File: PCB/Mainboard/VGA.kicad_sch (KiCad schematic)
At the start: 98 parts, among them J2 LCD_Connector, Q1 2SA1881-6, Q2 8C, U51 CHIPS65535

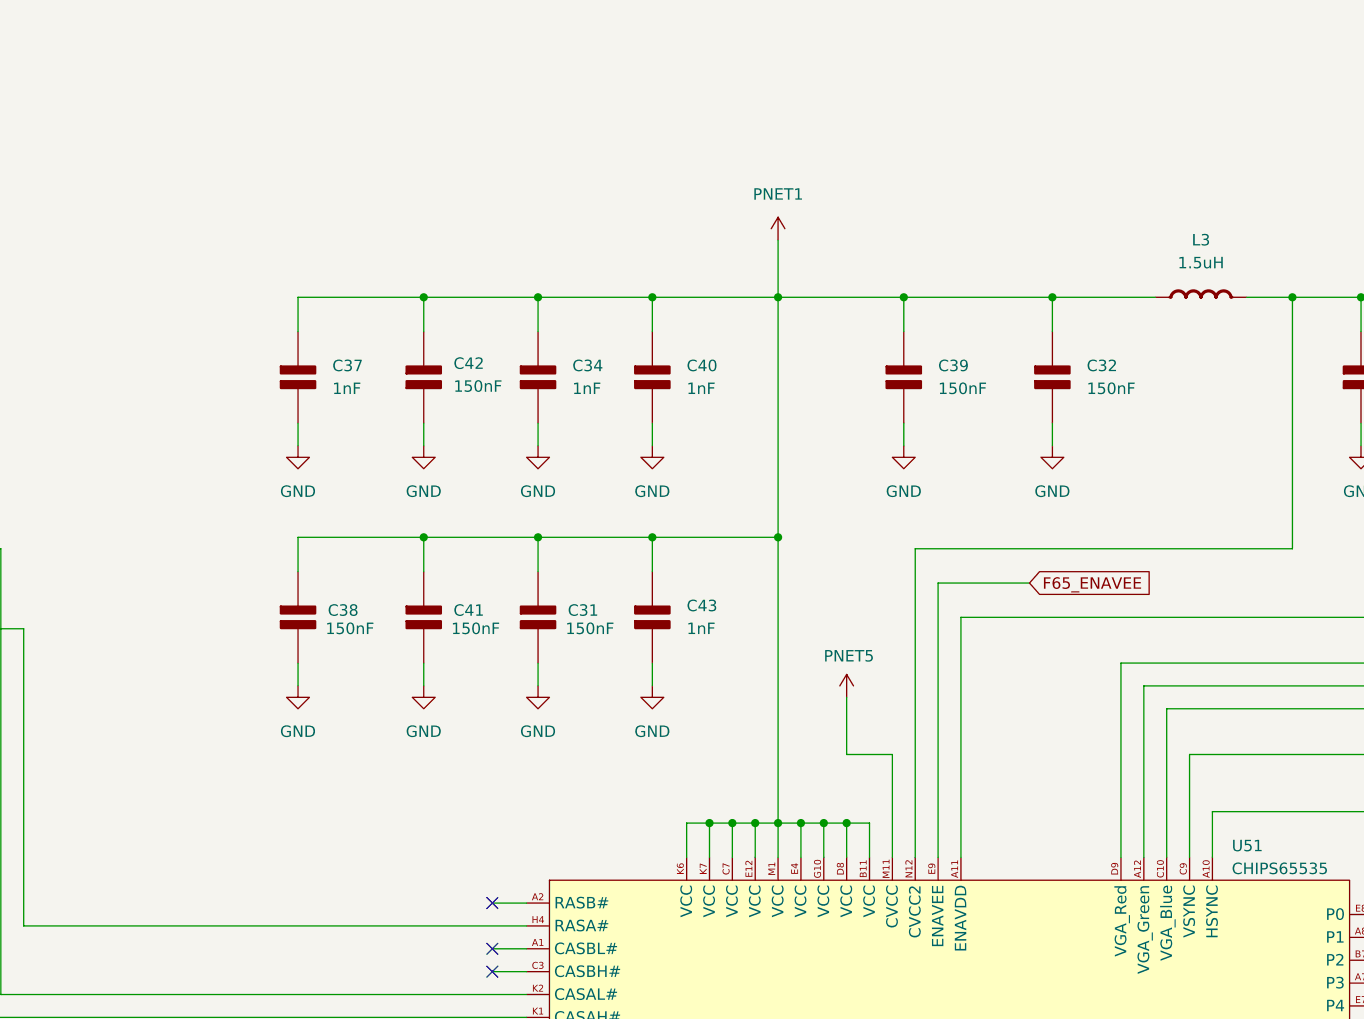
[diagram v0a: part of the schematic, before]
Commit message: Add files via upload
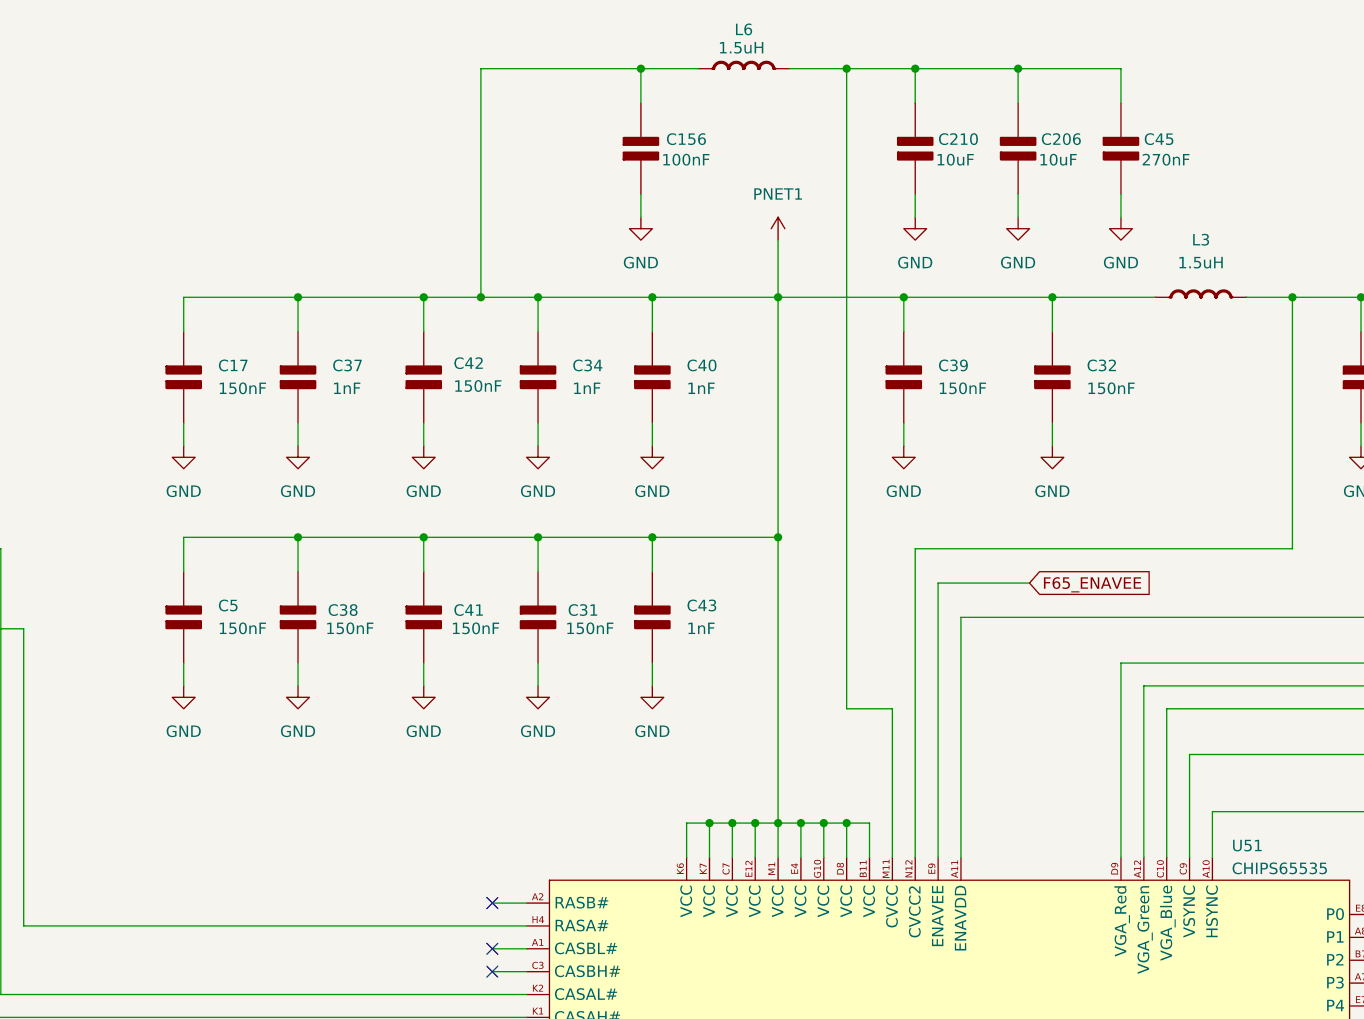
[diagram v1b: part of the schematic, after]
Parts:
- added C156: 100nF, symbol PCM_Elektuur:C
- added C17, C5: 150nF, symbol PCM_Elektuur:C
- added C206, C210: 10uF, symbol PCM_Elektuur:C
- added C45: 270nF, symbol PCM_Elektuur:C
- added L6: 1.5uH, symbol PCM_Elektuur:L
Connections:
- net GND: now also C156.1 (+), C17.2 (-), C206.2 (-), C210.2 (-), C45.2 (-), C5.2 (-)
- net PNET1: now also C156.2 (-), C17.1 (+), C5.1 (+), L6.2 (-)
- net PNET5: no longer U51.M11 (CVCC)
- new net: C206.1 (+), C210.1 (+), C45.1 (+), L6.1 (+), U51.M11 (CVCC)

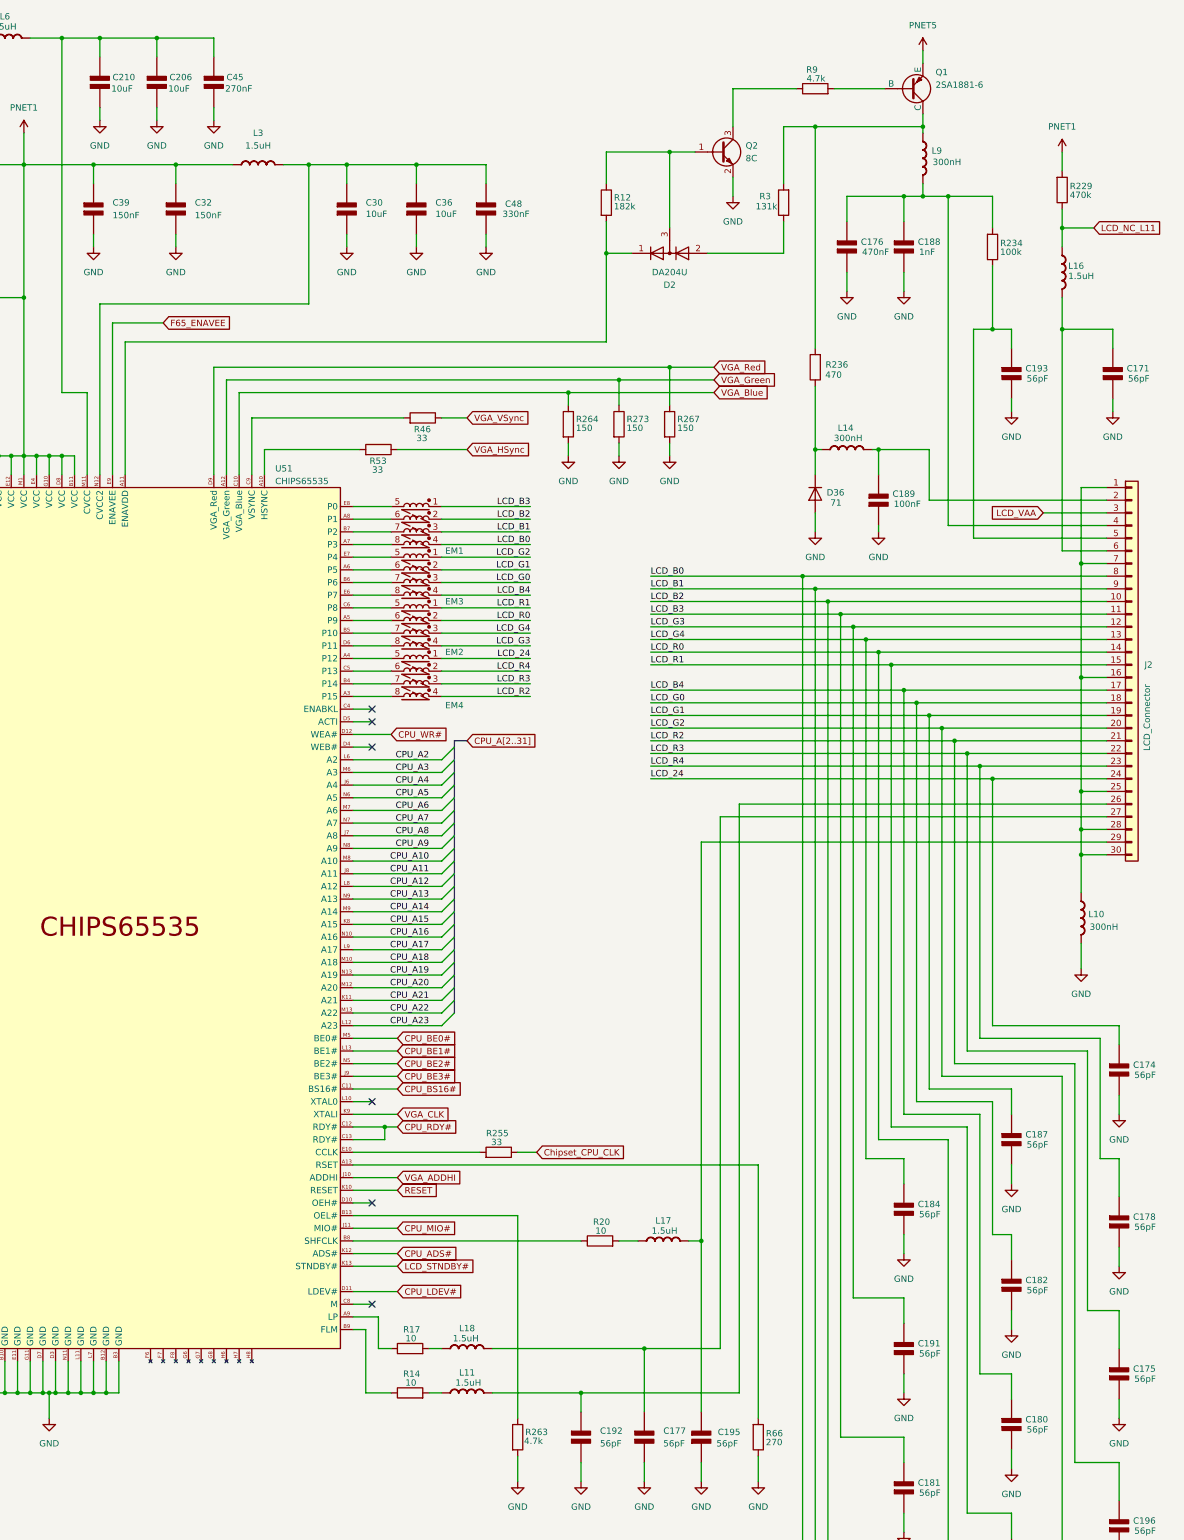
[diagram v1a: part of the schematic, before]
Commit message: Add files via upload
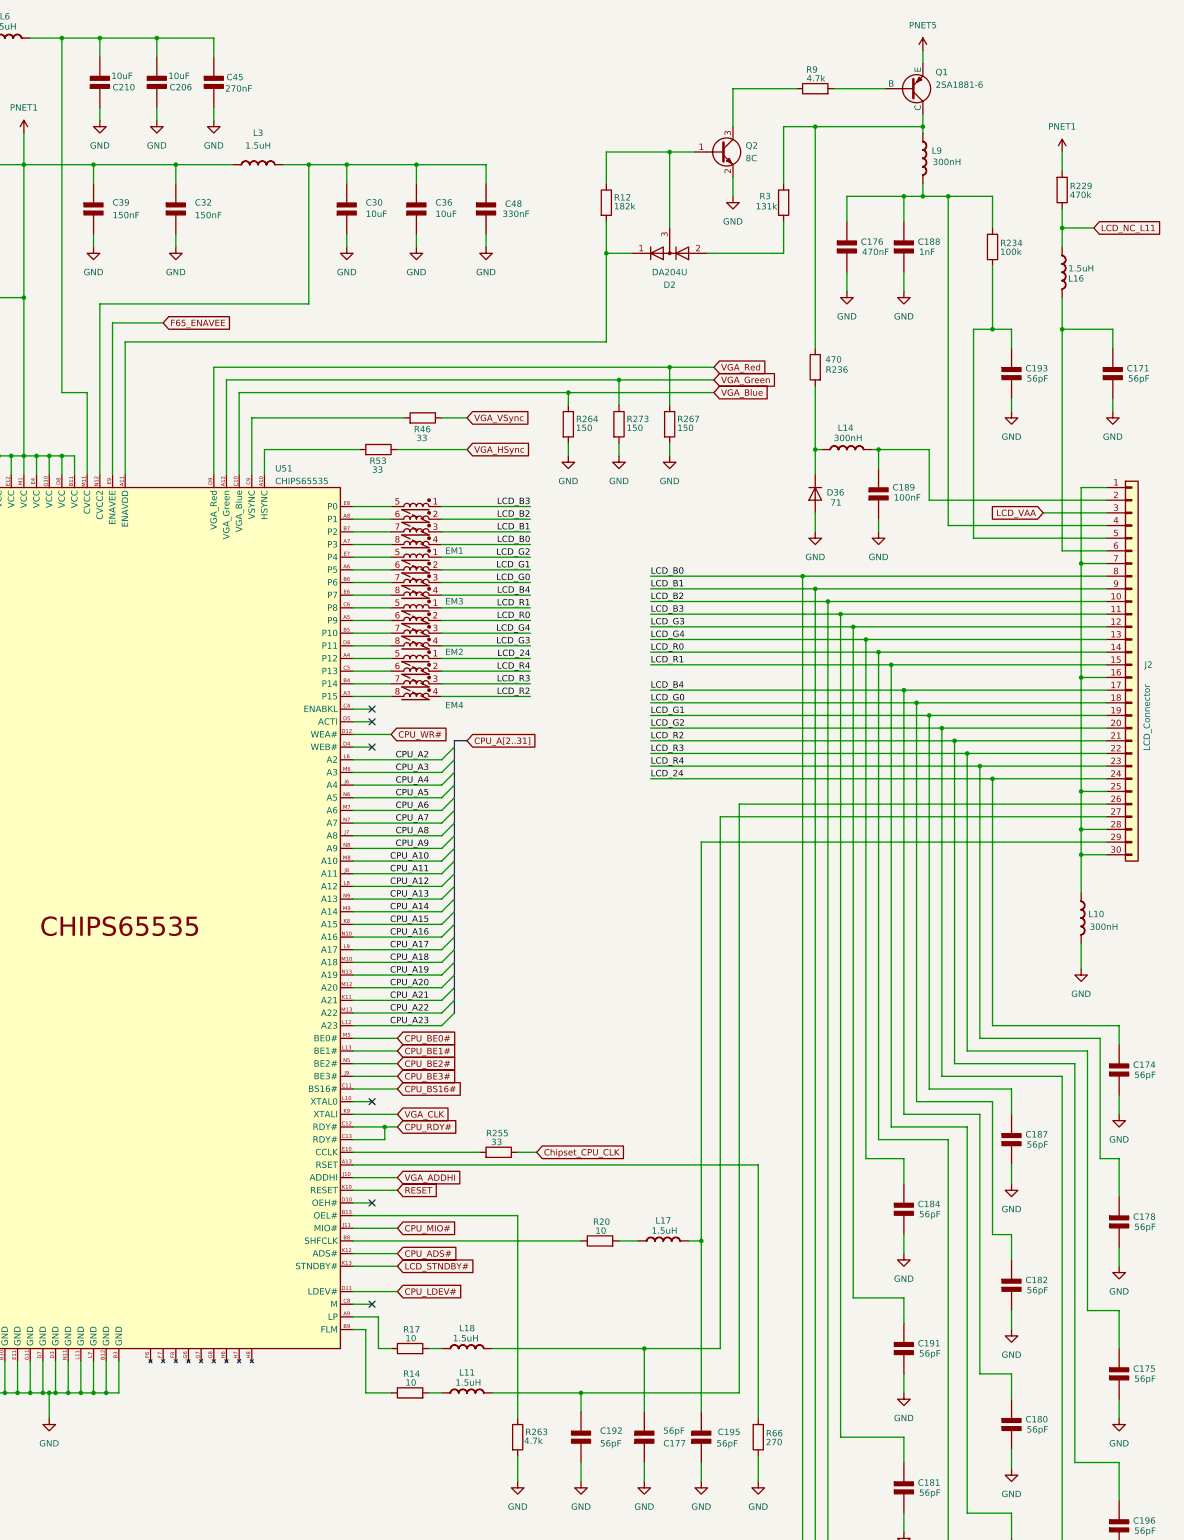
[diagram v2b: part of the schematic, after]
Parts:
- C156, C169, C17, C171, C172, C173, C174, C175, C177, C178, C180, C181, C182, C183, C184, C185, C186, C187, C188, C189, C191, C192, C193, C194, C195, C196, C26, C31, C32, C34, C37, C38, C39, C40, C41, C42, C43, C48, C5: footprint (none) -> Capacitor_SMD:C_0402_1005Metric
- C176, C45: footprint (none) -> Capacitor_SMD:C_0603_1608Metric
- C206, C210, C30, C36: footprint (none) -> Capacitor_SMD:C_1206_3216Metric
- D2: footprint (none) -> PC110:SOT-416L
- D36: footprint (none) -> Diode_SMD:D_0603_1608Metric
- EM1, EM2, EM3, EM4: footprint (none) -> PC110:R-array
- J2: footprint (none) -> PC110:LCD_connector
- L10, L9: footprint (none) -> Inductor_SMD:L_0805_2012Metric
- L11, L14, L16, L17, L18, L3, L6: footprint (none) -> Inductor_SMD:L_0603_1608Metric
- Q1: footprint (none) -> PCM_Package_TO_SOT_SMD_AKL:SOT-23
- Q2: footprint Package_TO_SOT_SMD:SOT-23 -> Package_TO_SOT_SMD:SOT-416
- R1, R10, R11, R12, R13, R14, R15, R16, R17, R18, R19, R2, R20, R21, R22, R229, R233, R234, R236, R255, R259, R263, R265, R269, R270, R279, R3, R46, R5, R51, R53, R58, R6, R61, R66, R7, R9: footprint (none) -> PCM_Resistor_SMD_AKL:R_0402_1005Metric
- R264, R267, R273: footprint (none) -> PCM_Resistor_SMD_AKL:R_0805_2012Metric
- U51: footprint (none) -> PC110:BGA-169
- U8: footprint (none) -> PC110:GRAMchip
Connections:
- net GND: now also C177.1 (+), C206.1 (+), C210.1 (+); no longer C177.2 (-), C206.2 (-), C210.2 (-)
- net LCD_NC_L11: now also L16.2 (-); no longer L16.1 (+)
- net at J2.27 (Pin_27), L18.1 (+): now also C177.2 (-); no longer C177.1 (+)
- net at D36.1 (K), L14.2 (-): now also R236.2; no longer R236.1
- net at L9.2 (-), Q1.1 (C), R3.2: now also R236.1; no longer R236.2
- net at C45.1 (+), L6.1 (+), U51.M11 (CVCC): now also C206.2 (-), C210.2 (-); no longer C206.1 (+), C210.1 (+)
- net at C171.1 (+), J2.6 (Pin_6): now also L16.1 (+); no longer L16.2 (-)
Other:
- moved on the sheet: C189, R236
